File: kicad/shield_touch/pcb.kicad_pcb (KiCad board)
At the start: 2 copper layers, 48.9 x 49.5 mm, 0 parts

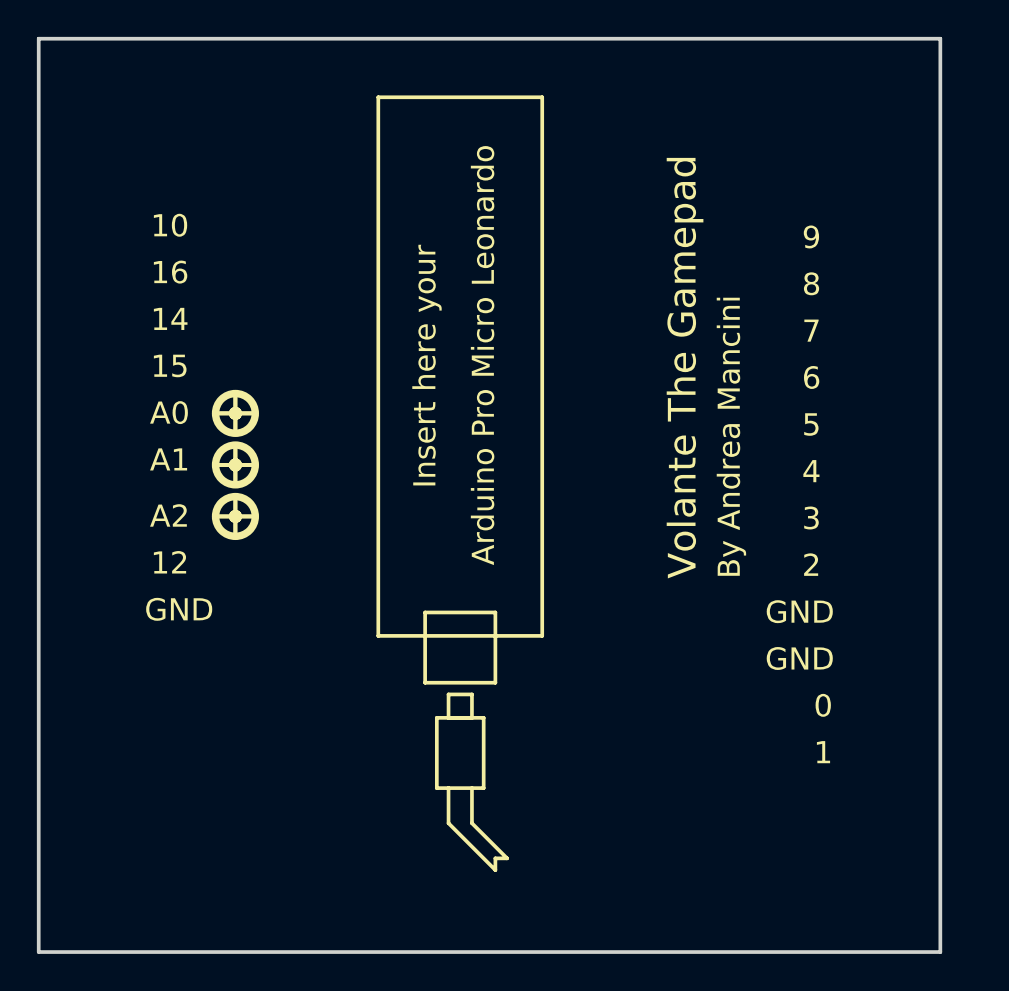
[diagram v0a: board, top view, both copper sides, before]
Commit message: update
- still to fix
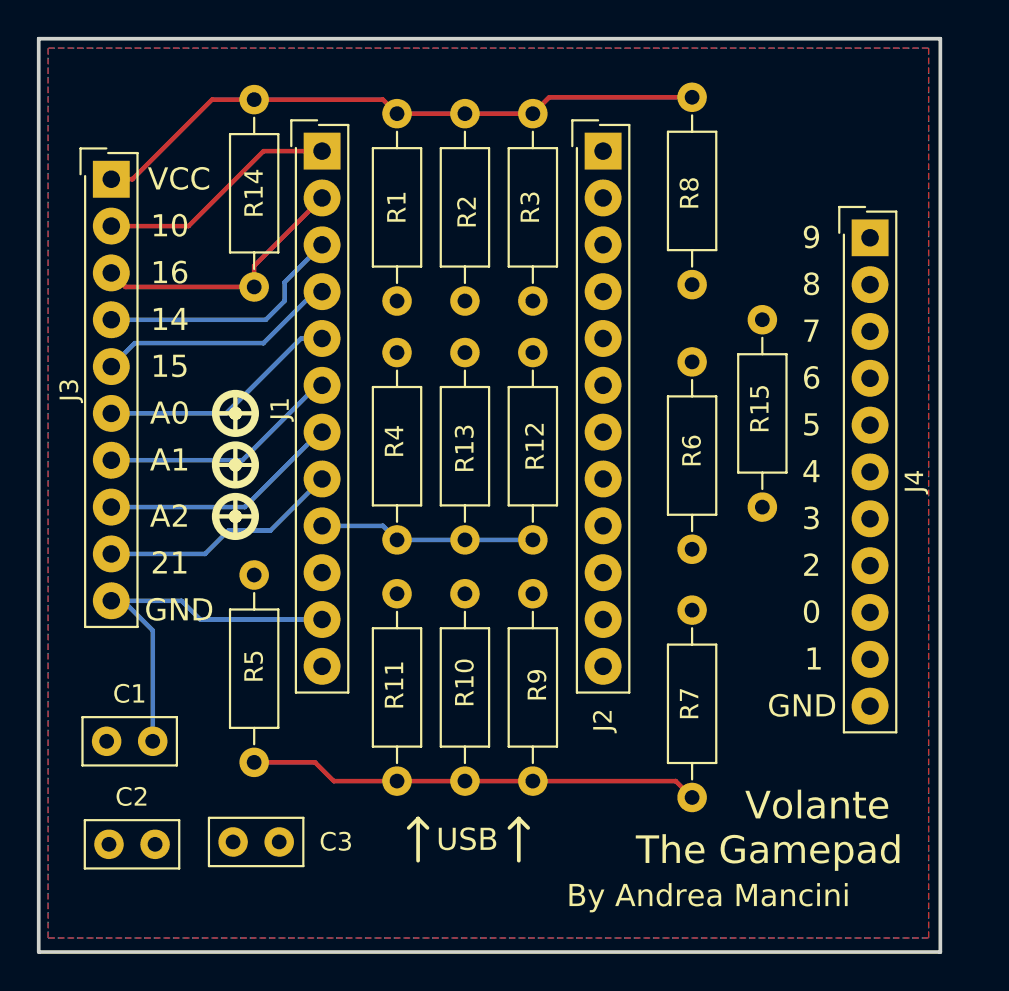
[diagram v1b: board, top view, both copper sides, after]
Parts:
- added C1: 0.01uF, Capacitors_THT:C_Disc_D5.0mm_W2.5mm_P2.50mm, F.Cu at (92.6, 99.1)
- added C2: 0.01uF, Capacitors_THT:C_Disc_D5.0mm_W2.5mm_P2.50mm, F.Cu at (92.7, 104.6)
- added C3: 0.01uF, Capacitors_THT:C_Disc_D5.0mm_W2.5mm_P2.50mm, F.Cu at (99.4, 104.5)
- added J1: Conn_01x12_Fem_l, Connectors_Samtec:SL-112-X-XX_1x12, F.Cu at (104.3, 67.1)
- added J2: Conn_01x12_Fem_r, Connectors_Samtec:SL-112-X-XX_1x12, F.Cu at (119.5, 67.1)
- added J3: Conn_01x09_Fem_b_l, Connectors_Samtec:SL-110-X-XX_1x10, F.Cu at (92.8, 68.6)
- added J4: Conn_01x11_Fem_b_r_touch, Connectors_Samtec:SL-111-X-XX_1x11, F.Cu at (134.0, 71.8)
- added R1: 2M, Resistors_THT:R_Axial_DIN0207_L6.3mm_D2.5mm_P10.16mm_Horizontal, F.Cu at (108.3, 65.0)
- added R10: 2M, Resistors_THT:R_Axial_DIN0207_L6.3mm_D2.5mm_P10.16mm_Horizontal, F.Cu at (112.0, 101.2)
- added R11: 2M, Resistors_THT:R_Axial_DIN0207_L6.3mm_D2.5mm_P10.16mm_Horizontal, F.Cu at (108.3, 101.2)
- added R12: 2M, Resistors_THT:R_Axial_DIN0207_L6.3mm_D2.5mm_P10.16mm_Horizontal, F.Cu at (115.7, 88.1)
- added R13: 2M, Resistors_THT:R_Axial_DIN0207_L6.3mm_D2.5mm_P10.16mm_Horizontal, F.Cu at (112.0, 88.1)
- added R14: 2M, Resistors_THT:R_Axial_DIN0207_L6.3mm_D2.5mm_P10.16mm_Horizontal, F.Cu at (100.6, 64.3)
- added R15: 2M, Resistors_THT:R_Axial_DIN0207_L6.3mm_D2.5mm_P10.16mm_Horizontal, F.Cu at (128.1, 86.4)
- added R2: 2M, Resistors_THT:R_Axial_DIN0207_L6.3mm_D2.5mm_P10.16mm_Horizontal, F.Cu at (112.0, 65.0)
- added R3: 2M, Resistors_THT:R_Axial_DIN0207_L6.3mm_D2.5mm_P10.16mm_Horizontal, F.Cu at (115.7, 65.0)
- added R4: 2M, Resistors_THT:R_Axial_DIN0207_L6.3mm_D2.5mm_P10.16mm_Horizontal, F.Cu at (108.3, 88.1)
- added R5: 2M, Resistors_THT:R_Axial_DIN0207_L6.3mm_D2.5mm_P10.16mm_Horizontal, F.Cu at (100.6, 100.2)
- added R6: 2M, Resistors_THT:R_Axial_DIN0207_L6.3mm_D2.5mm_P10.16mm_Horizontal, F.Cu at (124.3, 88.6)
- added R7: 2M, Resistors_THT:R_Axial_DIN0207_L6.3mm_D2.5mm_P10.16mm_Horizontal, F.Cu at (124.3, 102.1)
- added R8: 2M, Resistors_THT:R_Axial_DIN0207_L6.3mm_D2.5mm_P10.16mm_Horizontal, F.Cu at (124.3, 64.1)
- added R9: 2M, Resistors_THT:R_Axial_DIN0207_L6.3mm_D2.5mm_P10.16mm_Horizontal, F.Cu at (115.7, 101.2)
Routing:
- net VCC: track 0.00 -> 70.3 mm
- net GND: track 0.00 -> 20.8 mm
- net 16: track 0.00 -> 14.4 mm
- net 14: track 0.00 -> 13.7 mm
- net A0: track 0.00 -> 13.1 mm
- net 21: track 0.00 -> 13.1 mm
- net 10: track 0.00 -> 13.1 mm
- net 15: track 0.00 -> 13.1 mm
- net A2: track 0.00 -> 13.1 mm
- net A1: track 0.00 -> 13.1 mm
- added copper zone on B.Cu, net GND
- added copper zone on F.Cu, net GND
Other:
- board text added: "21"
- board text added: "USB"
- board text added: "VCC"
- board text removed: "12"
- board text removed: "Arduino Pro Micro Leonardo"
- board text removed: "Insert here your"
- board text removed: "Play your simulation games with"
- board text removed: "USB HID device Plug and Play Small and Cute :)"
- board text removed: "Volante"

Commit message: update
- still to fix
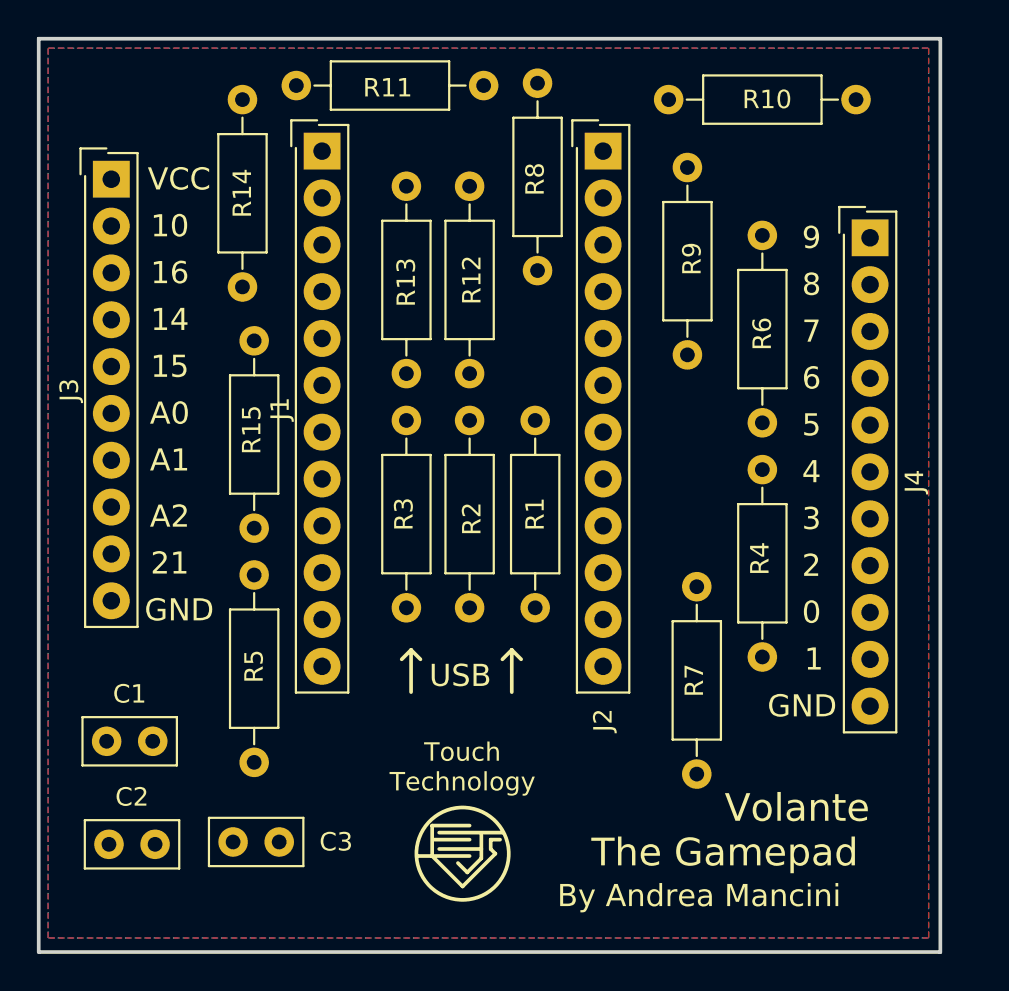
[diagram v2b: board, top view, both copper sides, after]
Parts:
- moved R10 38.6 mm to (123.1, 64.3), turned to 0 degrees
- moved R11 38.0 mm to (113.0, 63.5), turned to 180 degrees
- moved R15 27.6 mm to (100.6, 87.5)
- moved R9 24.6 mm to (124.1, 78.1)
- moved R4 20.8 mm to (128.1, 94.5)
- moved R1 18.2 mm to (115.8, 81.7)
- moved R3 18.0 mm to (108.8, 81.7)
- moved R6 17.4 mm to (128.1, 71.6), turned to 270 degrees
- moved R2 16.6 mm to (112.3, 81.7)
- moved R12 9.65 mm to (112.3, 79.1)
- moved R13 9.56 mm to (108.8, 79.1)
- moved R8 8.42 mm to (116.0, 63.4)
- moved R7 1.30 mm to (124.6, 100.8)
- moved R14 0.64 mm to (99.9, 64.3)
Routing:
- net VCC: track 70.3 -> 0.00 mm
- net GND: track 20.8 -> 0.00 mm
- net 16: track 14.4 -> 0.00 mm
- net 14: track 13.7 -> 0.00 mm
- net A0: track 13.1 -> 0.00 mm
- net 21: track 13.1 -> 0.00 mm
- net 10: track 13.1 -> 0.00 mm
- net A2: track 13.1 -> 0.13 mm
- net A1: track 13.1 -> 0.25 mm
- net 15: track 13.1 -> 0.38 mm
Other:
- board text added: "Touch Technology"

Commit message: update
- still working
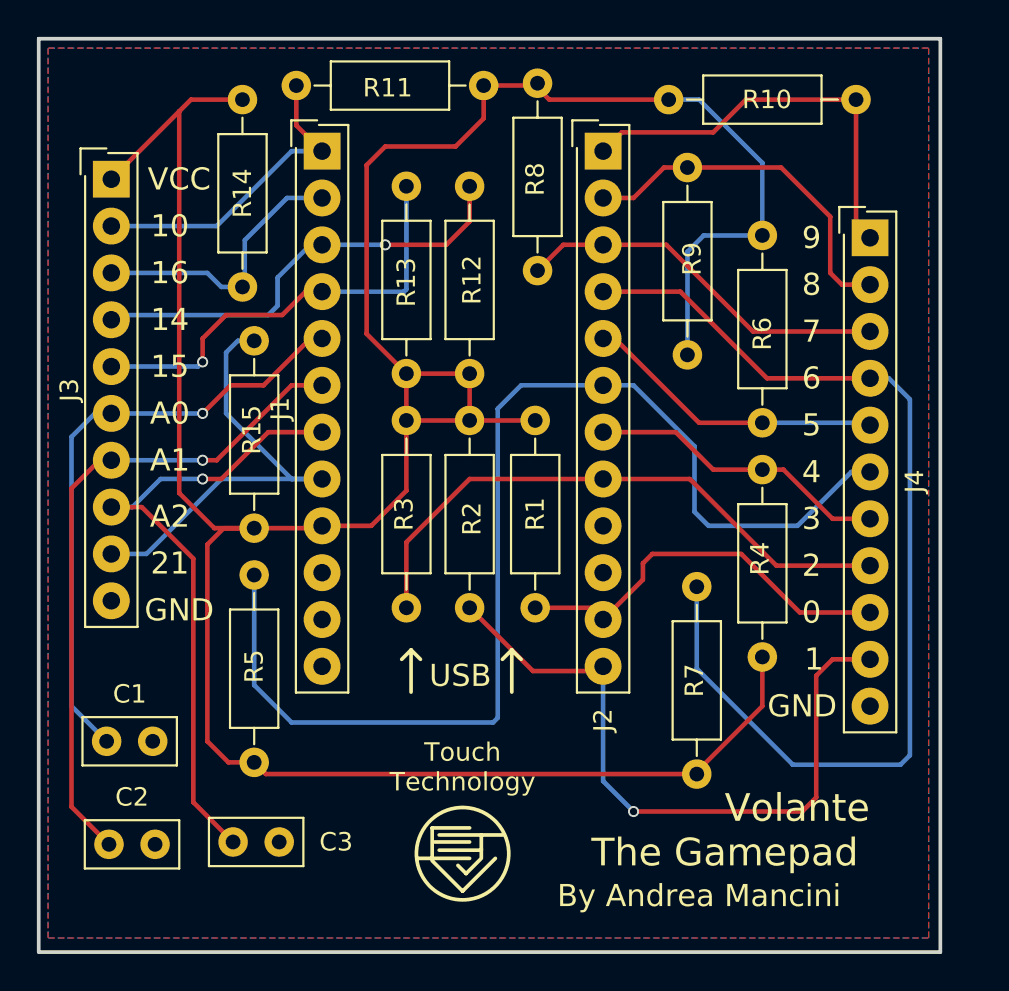
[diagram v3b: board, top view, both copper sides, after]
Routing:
- net VCC: track 0.00 -> 163.8 mm
- net 4: track 0.00 -> 64.1 mm
- net 6: track 0.00 -> 56.7 mm
- net 1: track 0.00 -> 37.4 mm, vias 0 -> 1
- net A1: track 0.25 -> 36.3 mm, vias 0 -> 1
- net A2: track 0.13 -> 35.1 mm, vias 0 -> 1
- net A0: track 0.00 -> 33.1 mm, vias 0 -> 1
- net 2: track 0.00 -> 32.1 mm
- net 21: track 0.00 -> 24.9 mm
- net 14: track 0.00 -> 24.4 mm, vias 0 -> 1
- net 15: track 0.38 -> 24.1 mm, vias 0 -> 1
- net 9: track 0.00 -> 22.7 mm
- net 0: track 0.00 -> 21.7 mm
- net 7: track 0.00 -> 20.6 mm
- net 8: track 0.00 -> 19.6 mm
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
